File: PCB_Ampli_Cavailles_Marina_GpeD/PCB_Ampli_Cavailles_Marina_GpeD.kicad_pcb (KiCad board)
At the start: 2 copper layers, 52 parts, among them J2 Conn_01x02, J3 Conn_01x03, Q1 2N2907, Q10 TIP32, Q11 BD138, Q12 TIP31, Q13 2N2222, Q2 2N2907, Q3 2N2907, Q4 2N2222, Q5 2N2222, Q6 2N2907, Q7 2N2907, Q8 BD139, Q9 BD139, U1 Relay_1CT, U2 Jack_Mono

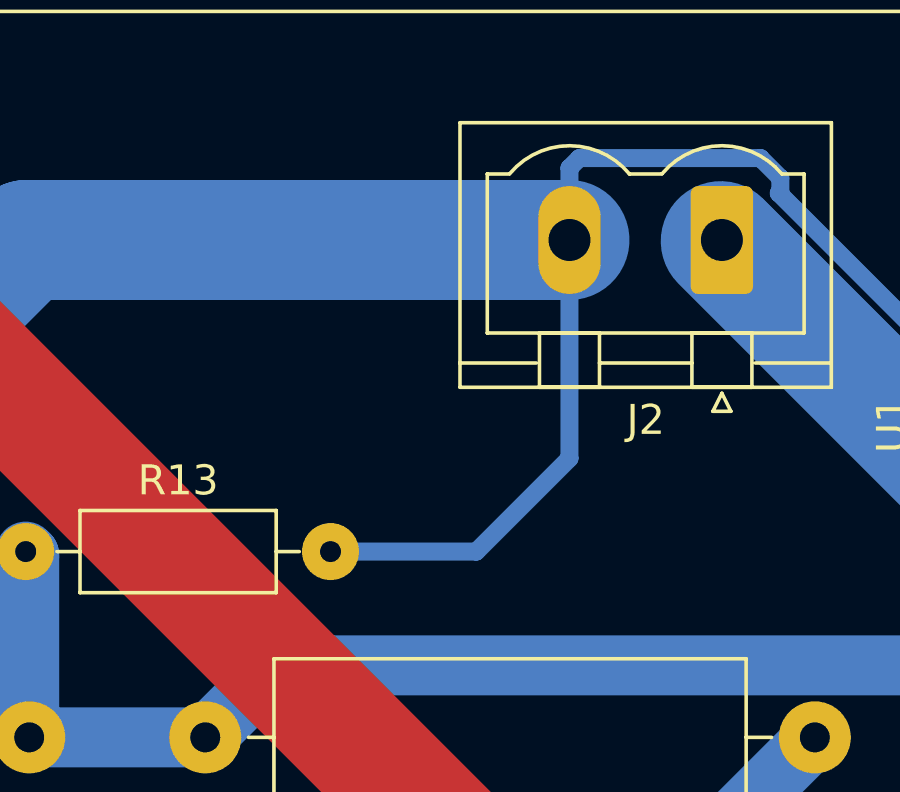
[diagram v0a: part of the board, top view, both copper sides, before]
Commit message: 4mm pour R13 à GND
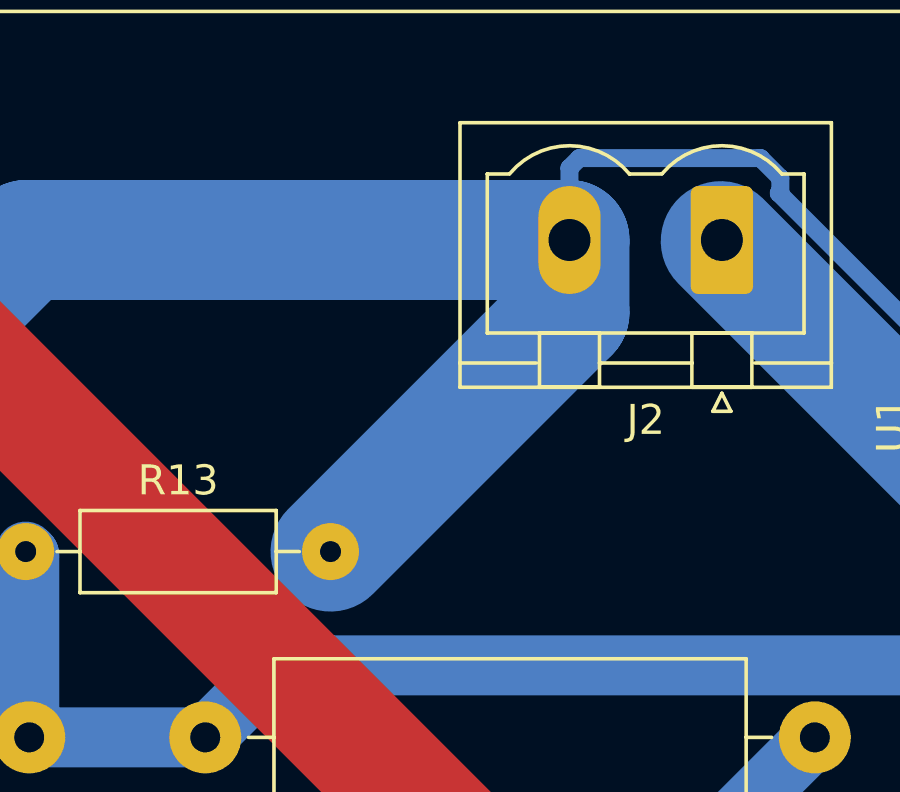
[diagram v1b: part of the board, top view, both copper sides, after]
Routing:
- net GND: track 405.4 -> 402.5 mm
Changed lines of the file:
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@@
     (thickness 1.6)
     (drawings 27)
-    (tracks 284)
+    (tracks 283)
     (zones 0)
     (modules 52)
@@
   )
   (setup
-    (last_trace_width 2)
+    (last_trace_width 4)
     (user_trace_width 0.6)
     (user_trace_width 1)
@@
   (segment (start 120.7421 40.62096) (end 120.00992 41.35314) (width 0.6) (layer B.Cu) (net 9))
   (segment (start 127.381 40.62096) (end 120.7421 40.62096) (width 0.6) (layer B.Cu) (net 9))
-  (segment (start 82.20456 43.40606) (end 87.06358 43.40606) (width 0.6) (layer B.Cu) (net 9))
-  (segment (start 90.17 40.29964) (end 90.17 33.02) (width 0.6) (layer B.Cu) (net 9))
-  (segment (start 87.06358 43.40606) (end 90.17 40.29964) (width 0.6) (layer B.Cu) (net 9))
   (segment (start 129.81686 43.05682) (end 127.381 40.62096) (width 0.6) (layer B.Cu) (net 9))
   (segment (start 129.81686 51.34102) (end 129.81686 43.05682) (width 0.6) (layer B.Cu) (net 9))
@@
   (segment (start 90.5005 30.2895) (end 90.17 30.62) (width 0.6) (layer B.Cu) (net 9))
   (segment (start 96.53778 30.2895) (end 90.5005 30.2895) (width 0.6) (layer B.Cu) (net 9))
+  (segment (start 90.17 35.44062) (end 82.20456 43.40606) (width 4) (layer B.Cu) (net 9))
+  (segment (start 90.17 33.02) (end 90.17 35.44062) (width 4) (layer B.Cu) (net 9))
   (segment (start 128.92278 89.949178) (end 132.60832 86.263638) (width 0.6) (layer B.Cu) (net 10))
   (segment (start 128.92278 91.29268) (end 128.92278 89.949178) (width 0.6) (layer B.Cu) (net 10))
